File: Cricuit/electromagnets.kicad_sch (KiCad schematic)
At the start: 30 parts, among them K1 Relay_SPST-NO, K10 Relay_SPST-NO, K2 Relay_SPST-NO, K3 Relay_SPST-NO, K4 Relay_SPST-NO, K5 Relay_SPST-NO, K6 Relay_SPST-NO, K7 Relay_SPST-NO, K8 Relay_SPST-NO, K9 Relay_SPST-NO

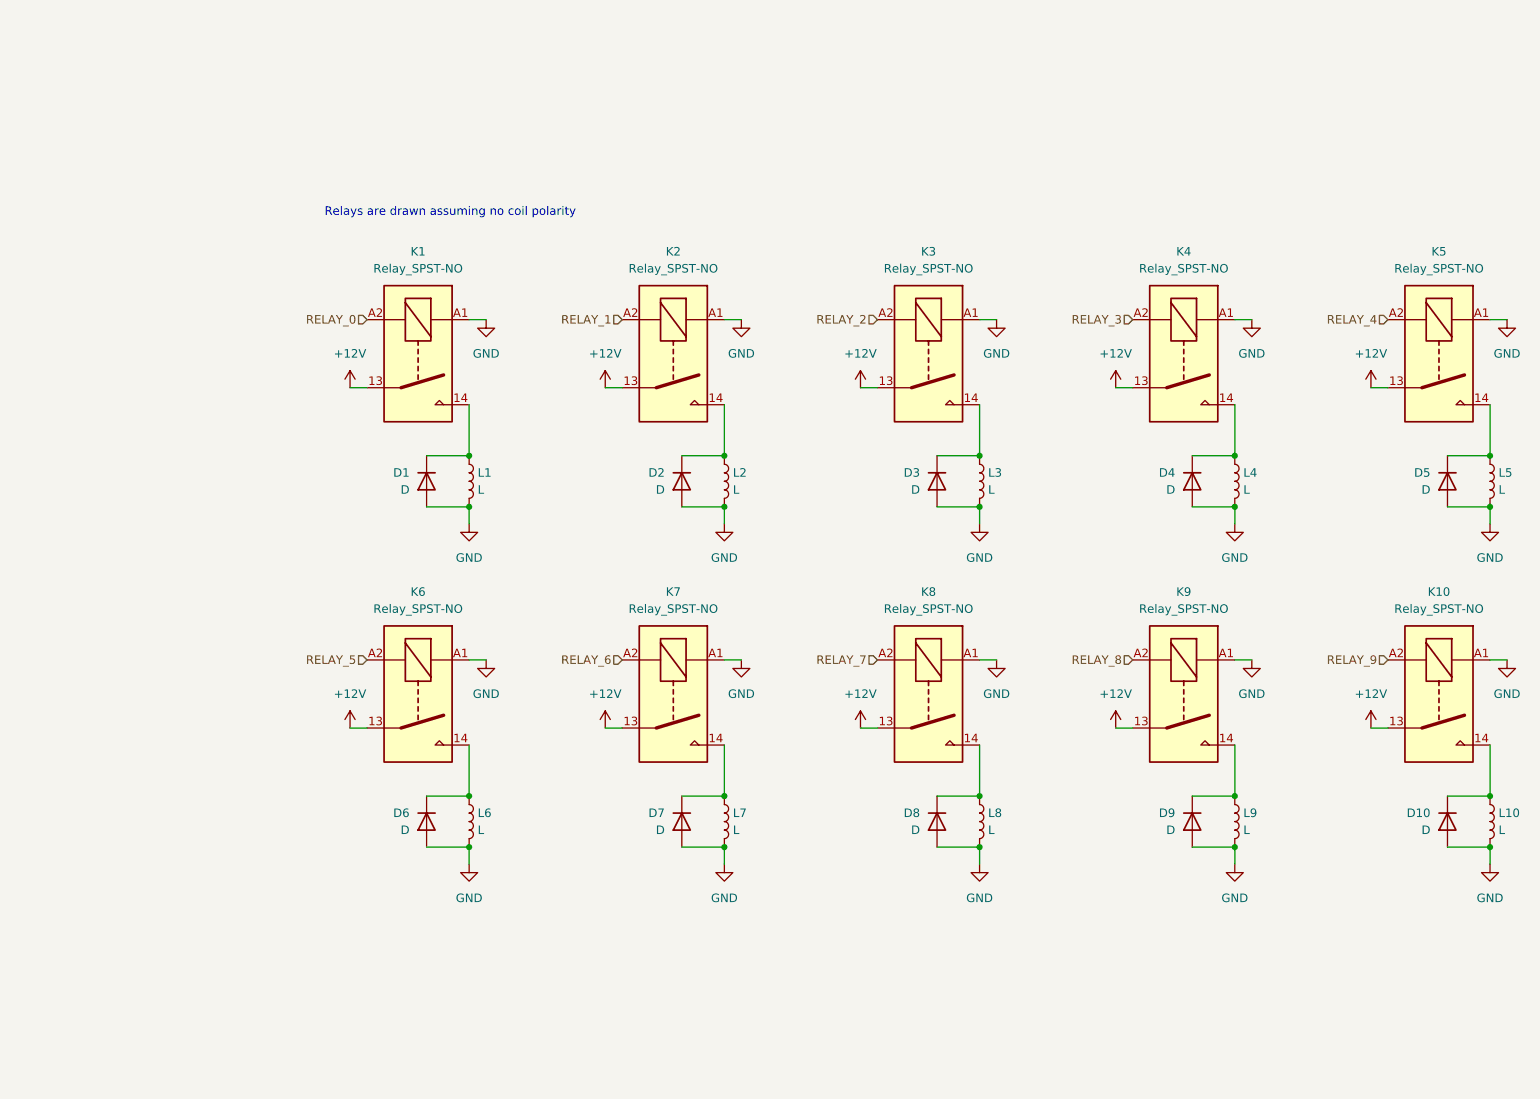
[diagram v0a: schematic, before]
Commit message: new stuff
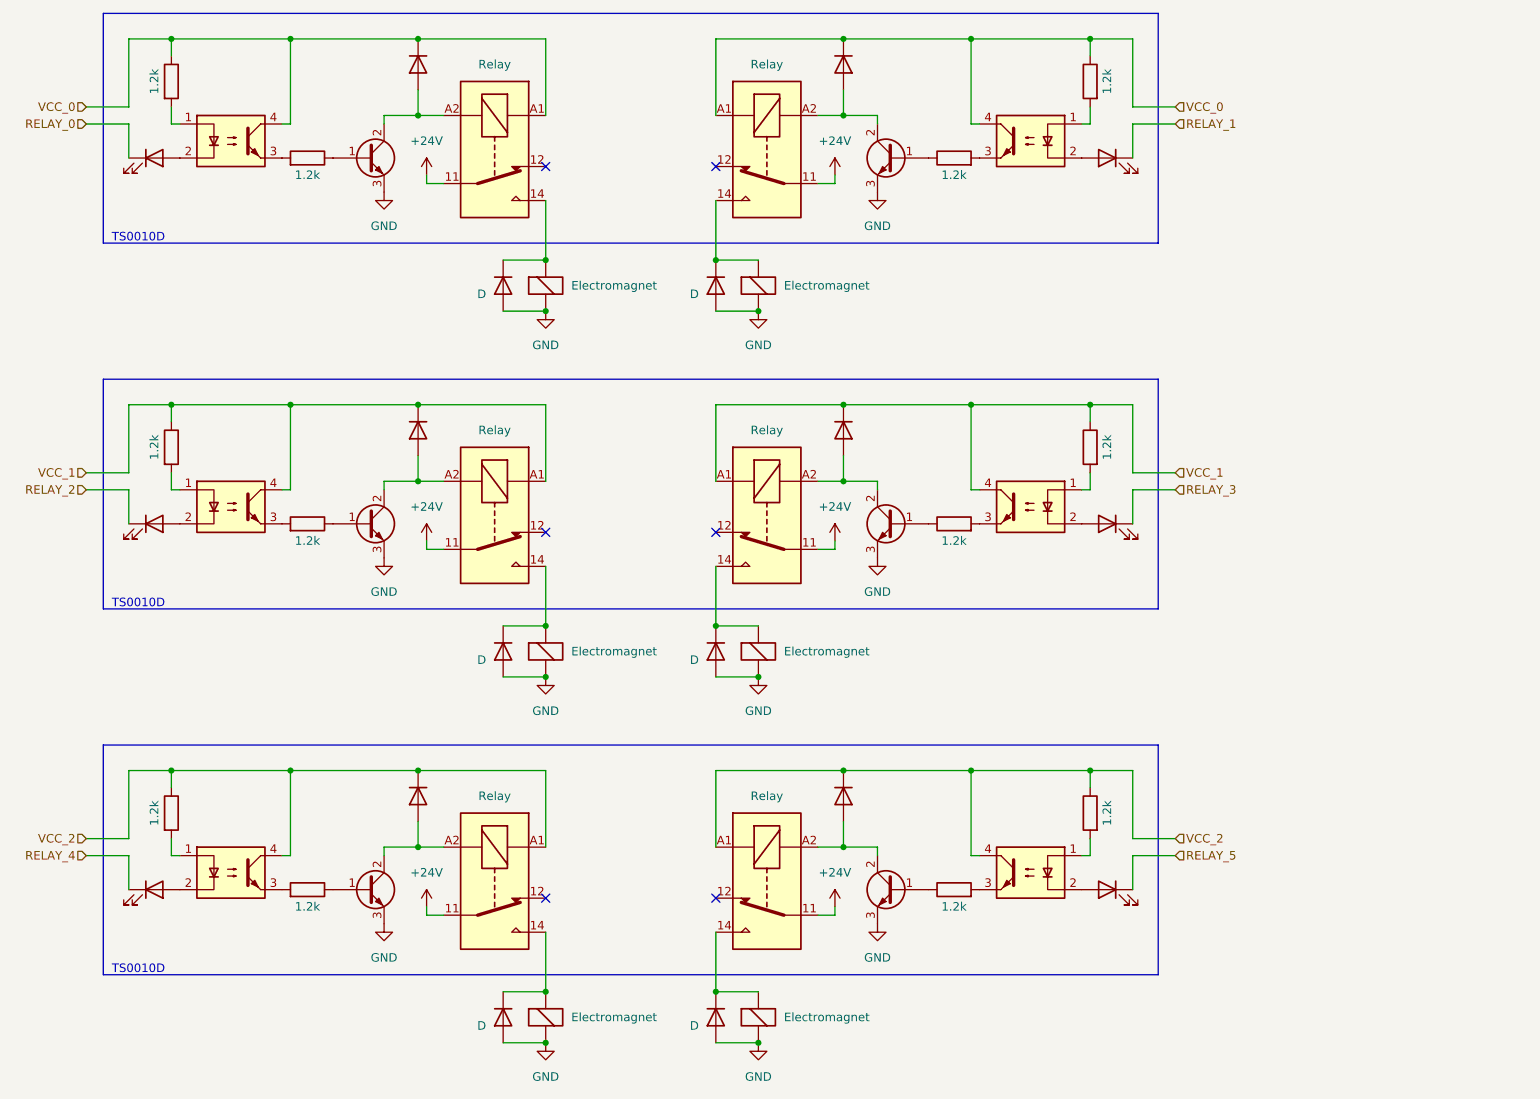
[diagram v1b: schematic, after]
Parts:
- removed D1, D10, D2, D3, D4, D5, D6, D7, D8, D9: D, symbol Device:D
- removed K1, K10, K2, K3, K4, K5, K6, K7, K8, K9: Relay_SPST-NO, symbol Relay:Relay_SPST-NO
- removed L1, L10, L2, L3, L4, L5, L6, L7, L8, L9: L, symbol Device:L
- added D301, D306, D307, D312, D313, D316: LED, symbol Device:LED
- added D302, D303, D304, D305, D308, D309, D310, D311, D314, D315, D317, D318: D, symbol Device:D
- added K301, K302, K303, K304, K305, K306: Relay, symbol Relay:Relay_SPDT
- added L301, L302, L303, L304, L305, L306: Electromagnet, symbol Device:ElectromagneticActor
- added Q301, Q302, Q303, Q304, Q305, Q306: Q_NPN_BCE, symbol Device:Q_NPN_BCE
- added R301, R302, R303, R304, R305, R306, R307, R308, R309, R310, R311, R312: 1.2k, symbol Device:R
- added U301, U302, U303, U304, U305, U306: EL817, Package_DIP:DIP-4_W7.62mm, symbol Isolator:EL817
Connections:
- net GND: now also D303.2 (A), D304.2 (A), D309.2 (A), D310.2 (A), D315.2 (A), D318.2 (A), L301.2 (+), L302.2 (+), L303.2 (+), L304.2 (+), L305.2 (+), L306.2 (+), Q301.3 (E), Q302.3 (E), Q303.3 (E), Q304.3 (E), Q305.3 (E), Q306.3 (E)
- net RELAY_0: now also D313.1 (K)
- net RELAY_1: now also D316.1 (K)
- net RELAY_2: now also D301.1 (K)
- net RELAY_3: now also D306.1 (K)
- net RELAY_4: now also D307.1 (K)
- net RELAY_5: now also D312.1 (K)
- new net: R311.2, U306.1
- new net: Q301.1 (B), R302.1
- new net: R302.2, U301.3
- new net: Q303.1 (B), R306.1
- new net: D308.2 (A), K303.A2, Q303.2 (C)
- new net: D311.2 (A), K304.A2, Q304.2 (C)
- new net: R309.2, U305.1
- new net: Q306.1 (B), R312.1
- new net: D317.2 (A), K306.A2, Q306.2 (C)
- new net: D304.1 (K), K302.14, L302.1 (-)
- new net: Q304.1 (B), R307.1
- new net: D309.1 (K), K303.14, L303.1 (-)
- new net: R301.2, U301.1
- new net: D301.2 (A), U301.2
- new net: R306.2, U303.3
- new net: D314.2 (A), K305.A2, Q305.2 (C)
- new net: D303.1 (K), K301.14, L301.1 (-)
- new net: D302.2 (A), K301.A2, Q301.2 (C)
- new net: D318.1 (K), K306.14, L306.1 (-)
- new net: R307.2, U304.3
- new net: D306.2 (A), U302.2
- new net: D316.2 (A), U306.2
- new net: D310.1 (K), K304.14, L304.1 (-)
- new net: R305.2, U303.1
- new net: D307.2 (A), U303.2
- new net: R312.2, U306.3
- new net: D315.1 (K), K305.14, L305.1 (-)
- new net: D305.2 (A), K302.A2, Q302.2 (C)
- new net: D312.2 (A), U304.2
- new net: R304.2, U302.1
- new net: Q305.1 (B), R310.1
- new net: R308.2, U304.1
- new net: R310.2, U305.3
- new net: R303.2, U302.3
- new net: D313.2 (A), U305.2
- new net: Q302.1 (B), R303.1
- new net +24V: K301.11, K302.11, K303.11, K304.11, K305.11, K306.11
- new net VCC_0: D314.1 (K), D317.1 (K), K305.A1, K306.A1, R309.1, R311.1, U305.4, U306.4
- new net VCC_1: D302.1 (K), D305.1 (K), K301.A1, K302.A1, R301.1, R304.1, U301.4, U302.4
- new net VCC_2: D308.1 (K), D311.1 (K), K303.A1, K304.A1, R305.1, R308.1, U303.4, U304.4
- no-connect marks 0 -> 6
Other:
- note added: "TS0010D"
- note removed: "Relays are drawn assuming no coil polarity"
